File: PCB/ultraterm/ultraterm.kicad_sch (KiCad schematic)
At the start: 13 parts, among them J1 ILI9341, J2 Battery_plug, J3 SD_Card_Receptacle, J4 SD_Card_Device, J5 Micro_SD_Card, SW1 SW_Push, SW2 SW_Push, SW3 SW_Push, SW4 SW_SPST, U2 LM809

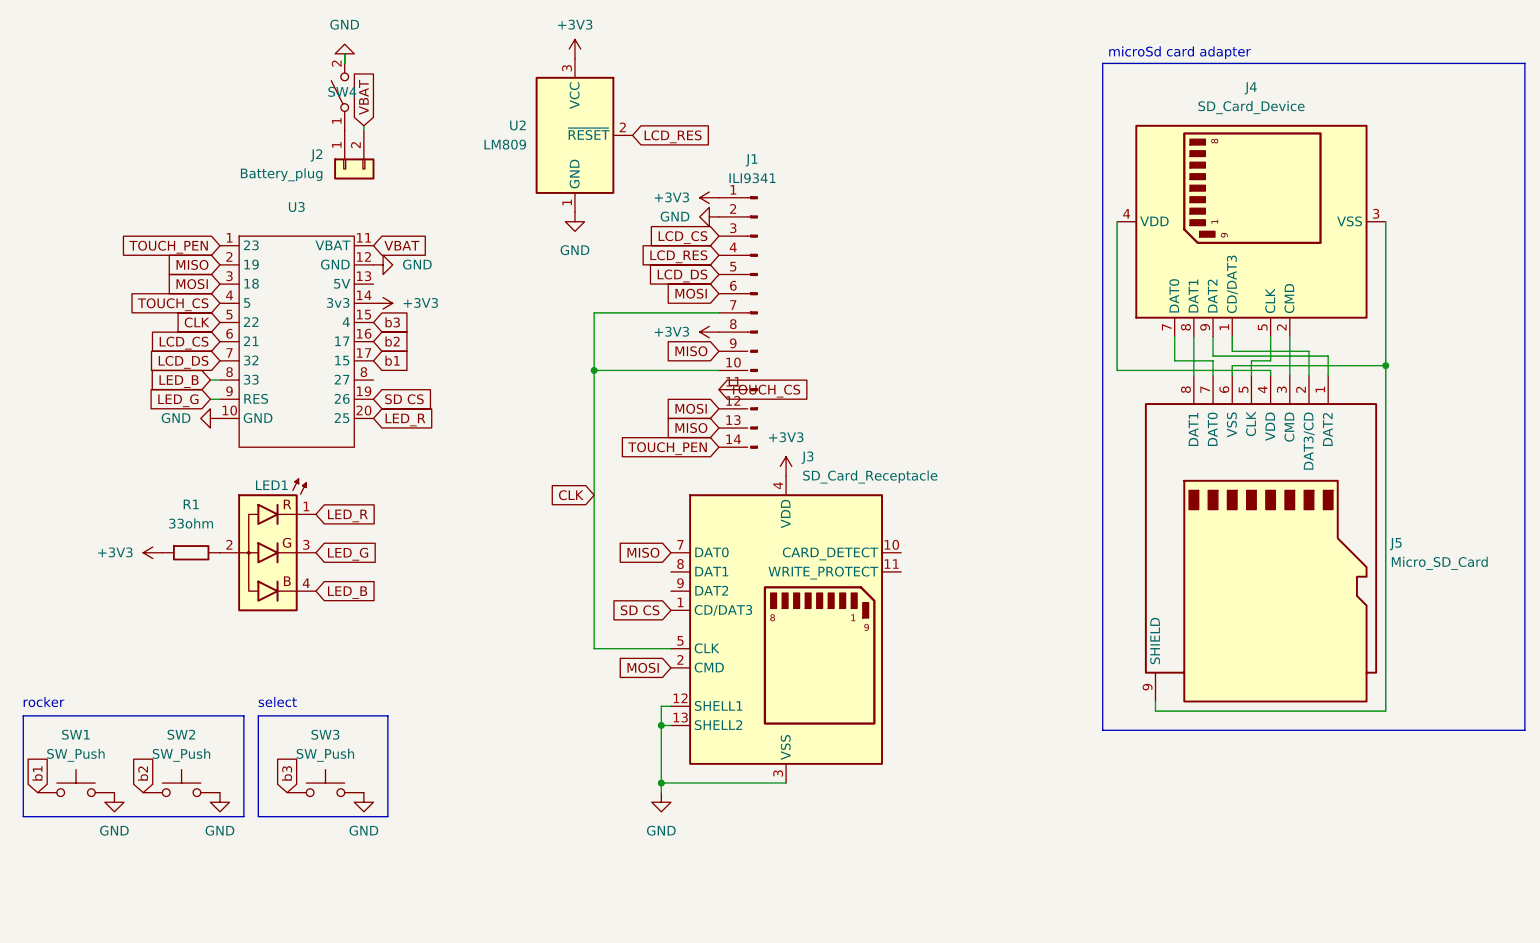
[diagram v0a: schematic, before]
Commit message: Final beta firmware.
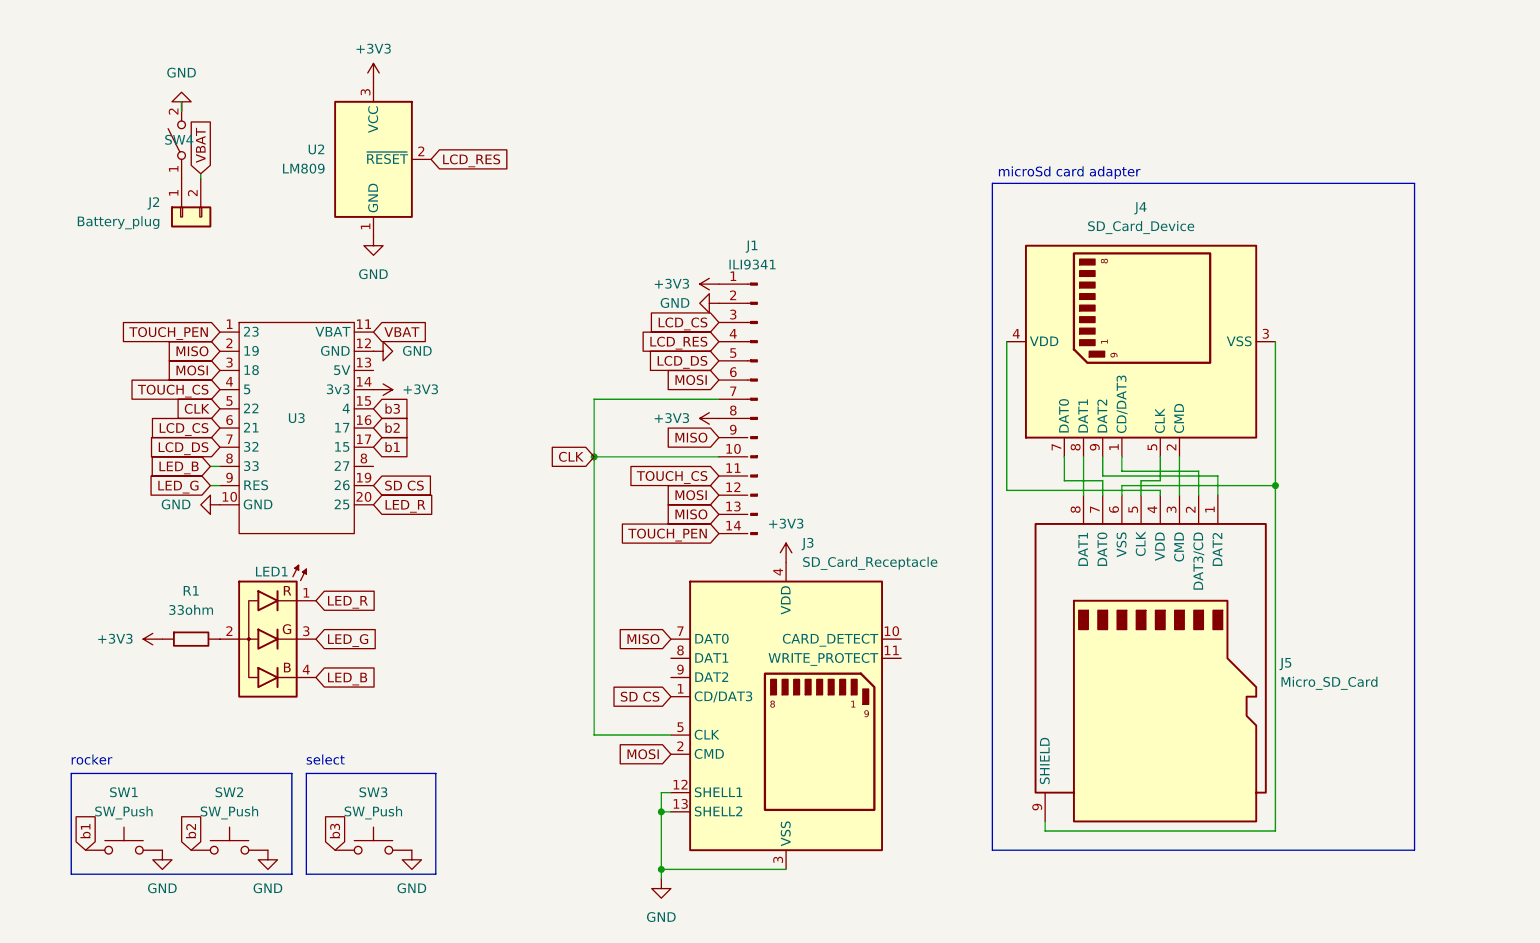
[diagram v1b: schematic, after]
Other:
- moved on the sheet: J1, J2, J3, J4, J5, LED1, R1, SW1, SW2, SW3, SW4, U2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
